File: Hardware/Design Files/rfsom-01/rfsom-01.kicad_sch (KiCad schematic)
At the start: 7 parts, among them J1 TC2050, J2 1054550101

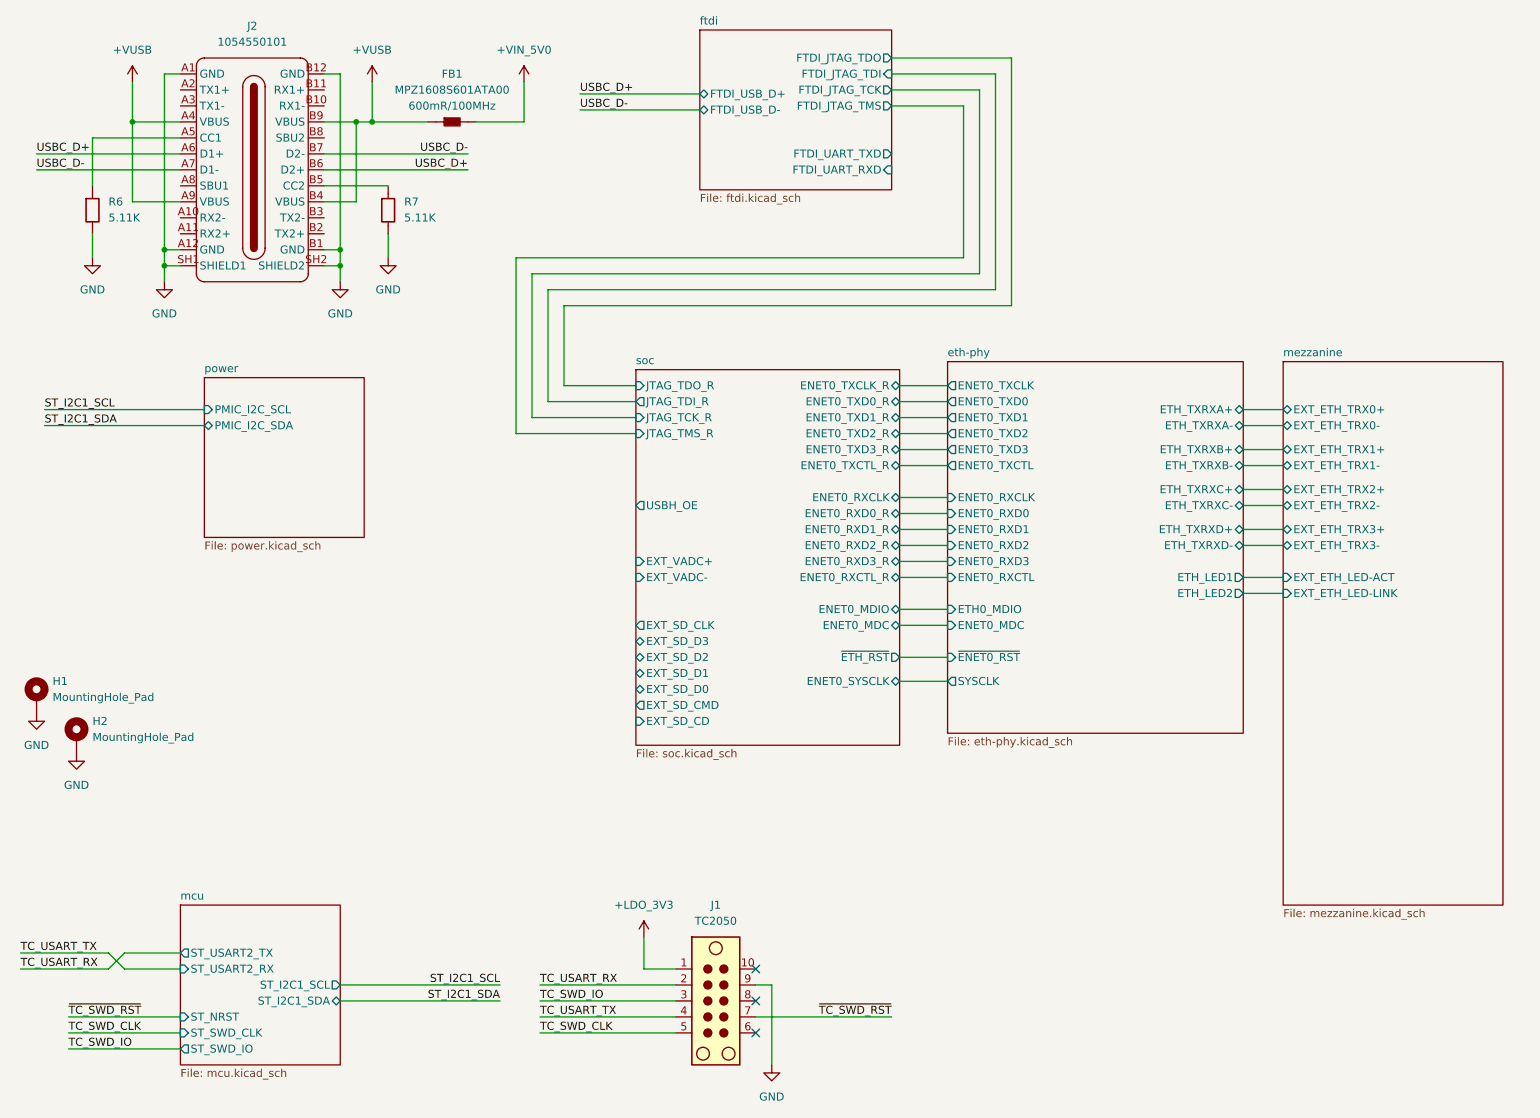
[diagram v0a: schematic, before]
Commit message: added starage, usb sch; more design progress in sch;
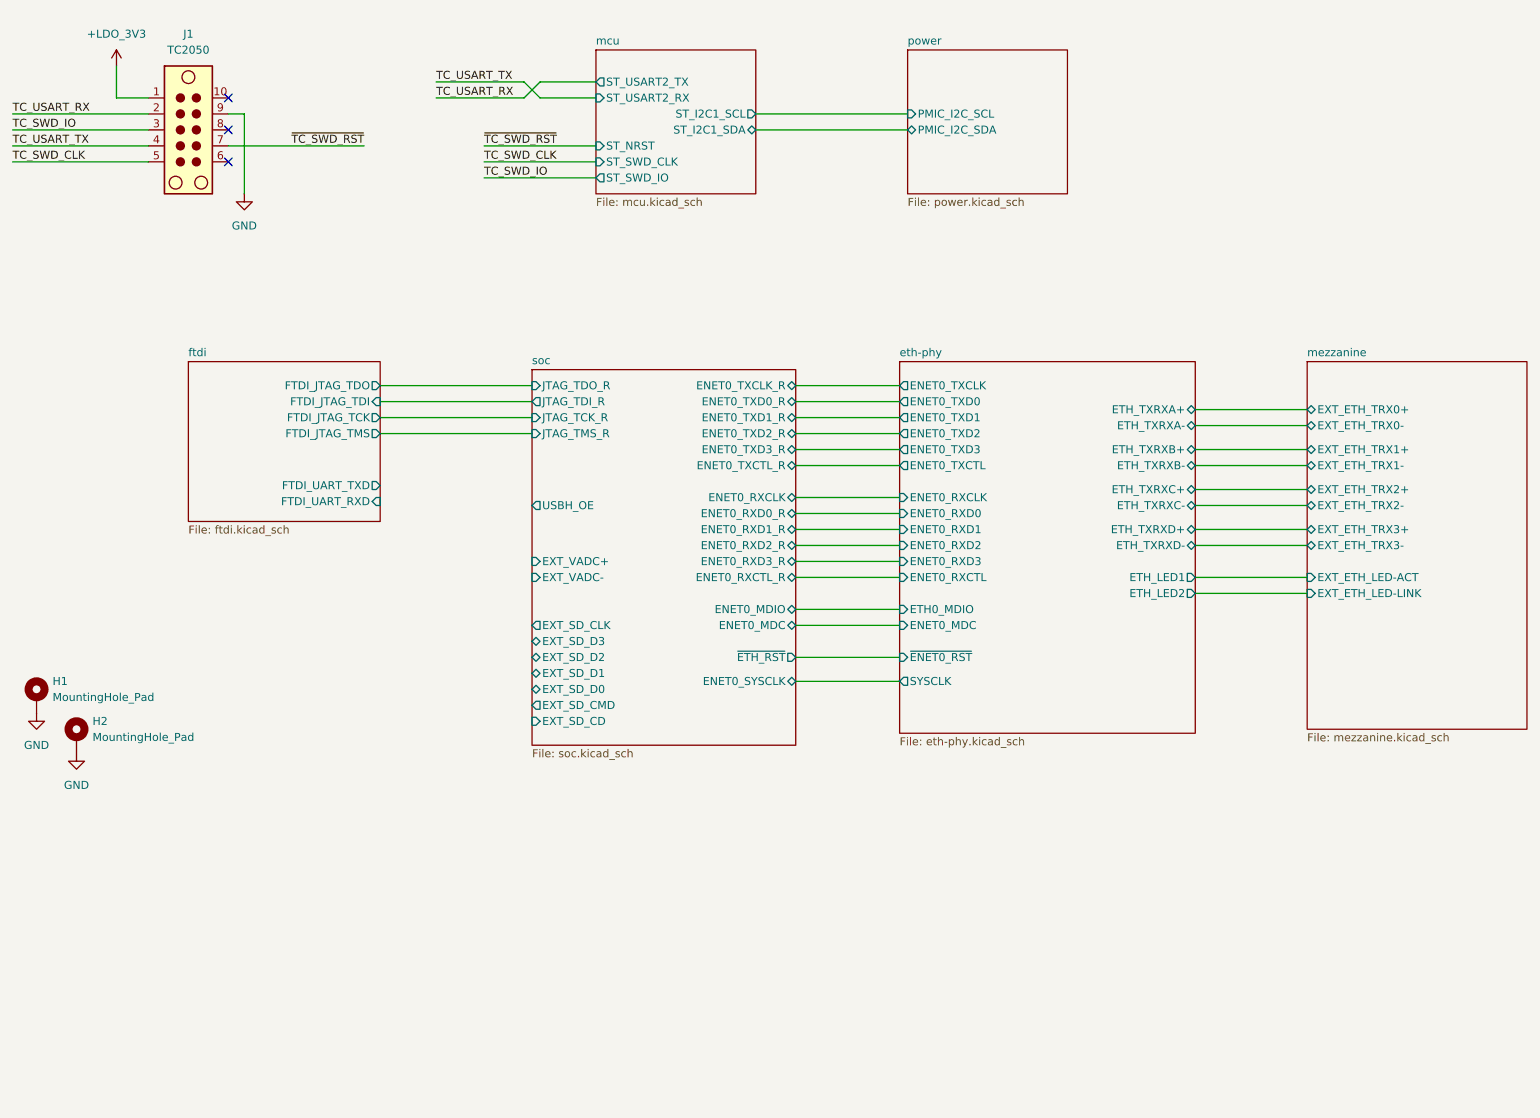
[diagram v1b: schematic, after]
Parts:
- removed FB1: MPZ1608S601ATA00, Resistor_SMD:R_0603_1608Metric, symbol Inductors:MPZ1608S601ATA00
- removed J2: 1054550101, Connectors:1054550101, symbol Connectors:1054550101
- removed R6, R7: RC0603FR-135K11L, Resistor_SMD:R_0603_1608Metric, symbol Resistors:RC0603FR-135K11L
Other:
- sheet ftdi ports: added none; removed FTDI_USB_D+, FTDI_USB_D-
- moved on the sheet: J1
